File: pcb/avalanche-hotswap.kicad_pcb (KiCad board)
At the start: 2 copper layers, 179.4 x 122.8 mm, 138 parts, among them J1 TRRS, J2 OLED, P1 i2c_pin, P2 i2c_pin, P3 battery+, P4 battery-, SW0 SW_Push, SW1 SW_Push, SW10 SW_Push, SW11 SW_Push, SW12 SW_Push, SW13 SW_Push, SW14 SW_Push, SW15 SW_Push, SW16 SW_Push, SW17 SW_Push, SW18 SW_Push, SW19 SW_Push, SW2 SW_Push, SW20 SW_Push, SW21 SW_Push, SW22 SW_Push, SW23 SW_Push, SW24 SW_Push, SW25 SW_Push, SW26 SW_Push, SW27 SW_Push, SW28 SW_Push, SW29 SW_Push, SW3 SW_Push, SW30 SW_Push, SW31 SW_Push, SW32 SW_Push, SW33 SW_DPDT_x2, SW34 SW_DPDT_x2, SW4 SW_Push, SW5 SW_Push, SW6 SW_Push, SW7 SW_Push, SW8 SW_Push, SW9 SW_Push, U1 ProMicro

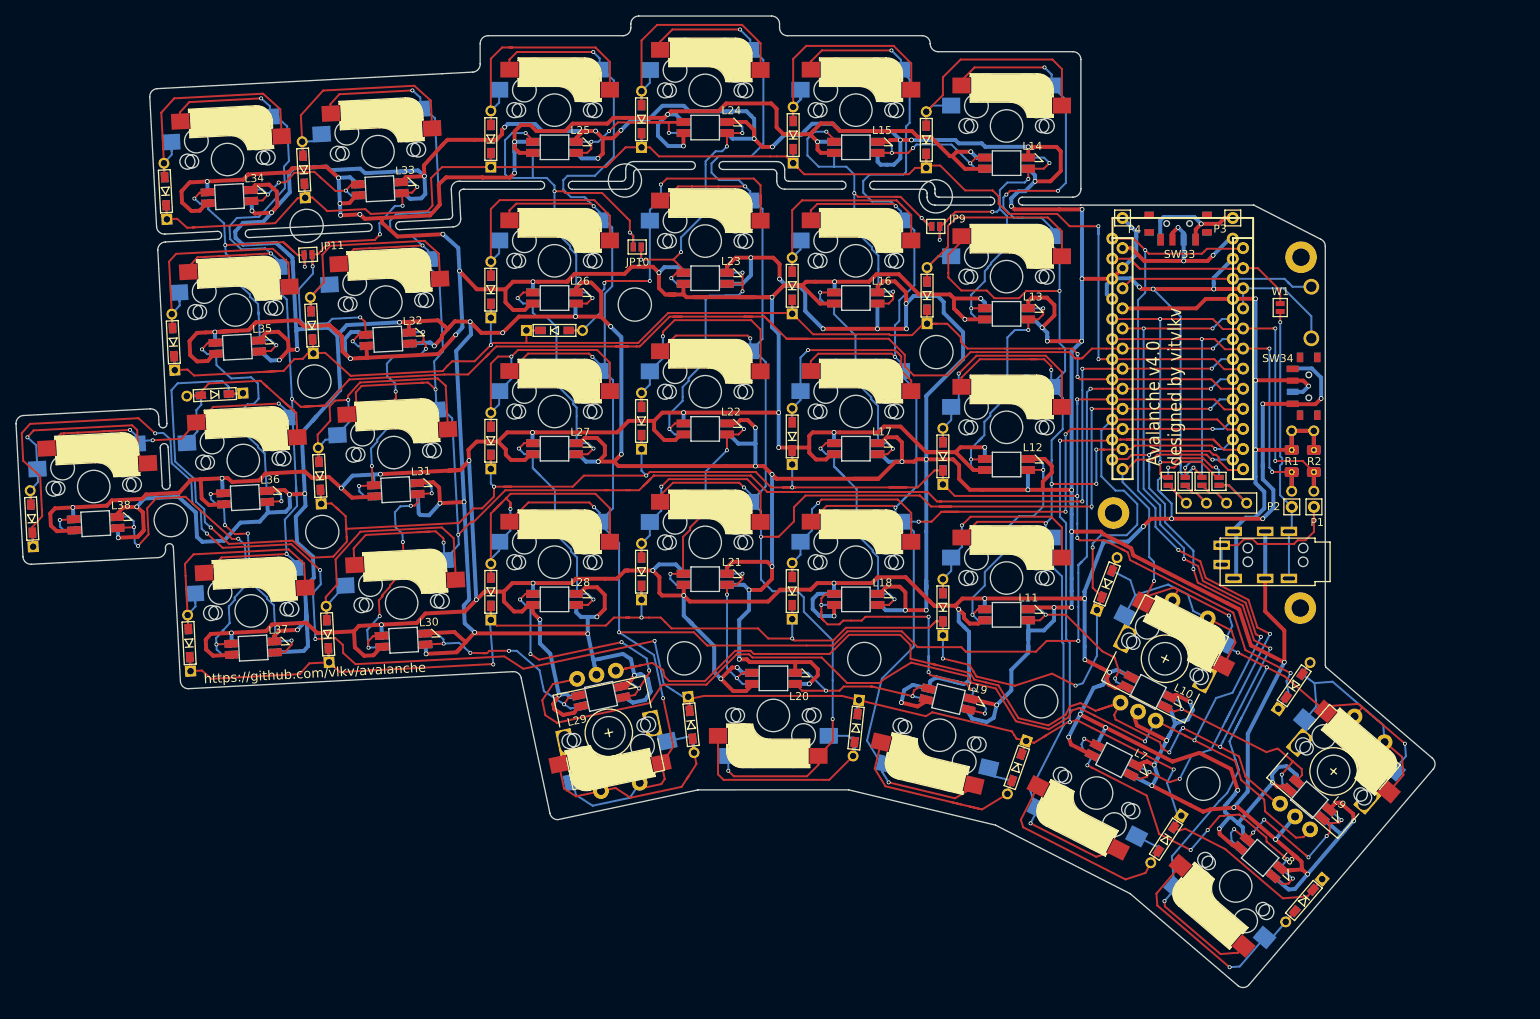
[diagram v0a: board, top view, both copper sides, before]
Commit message: Working on stagger
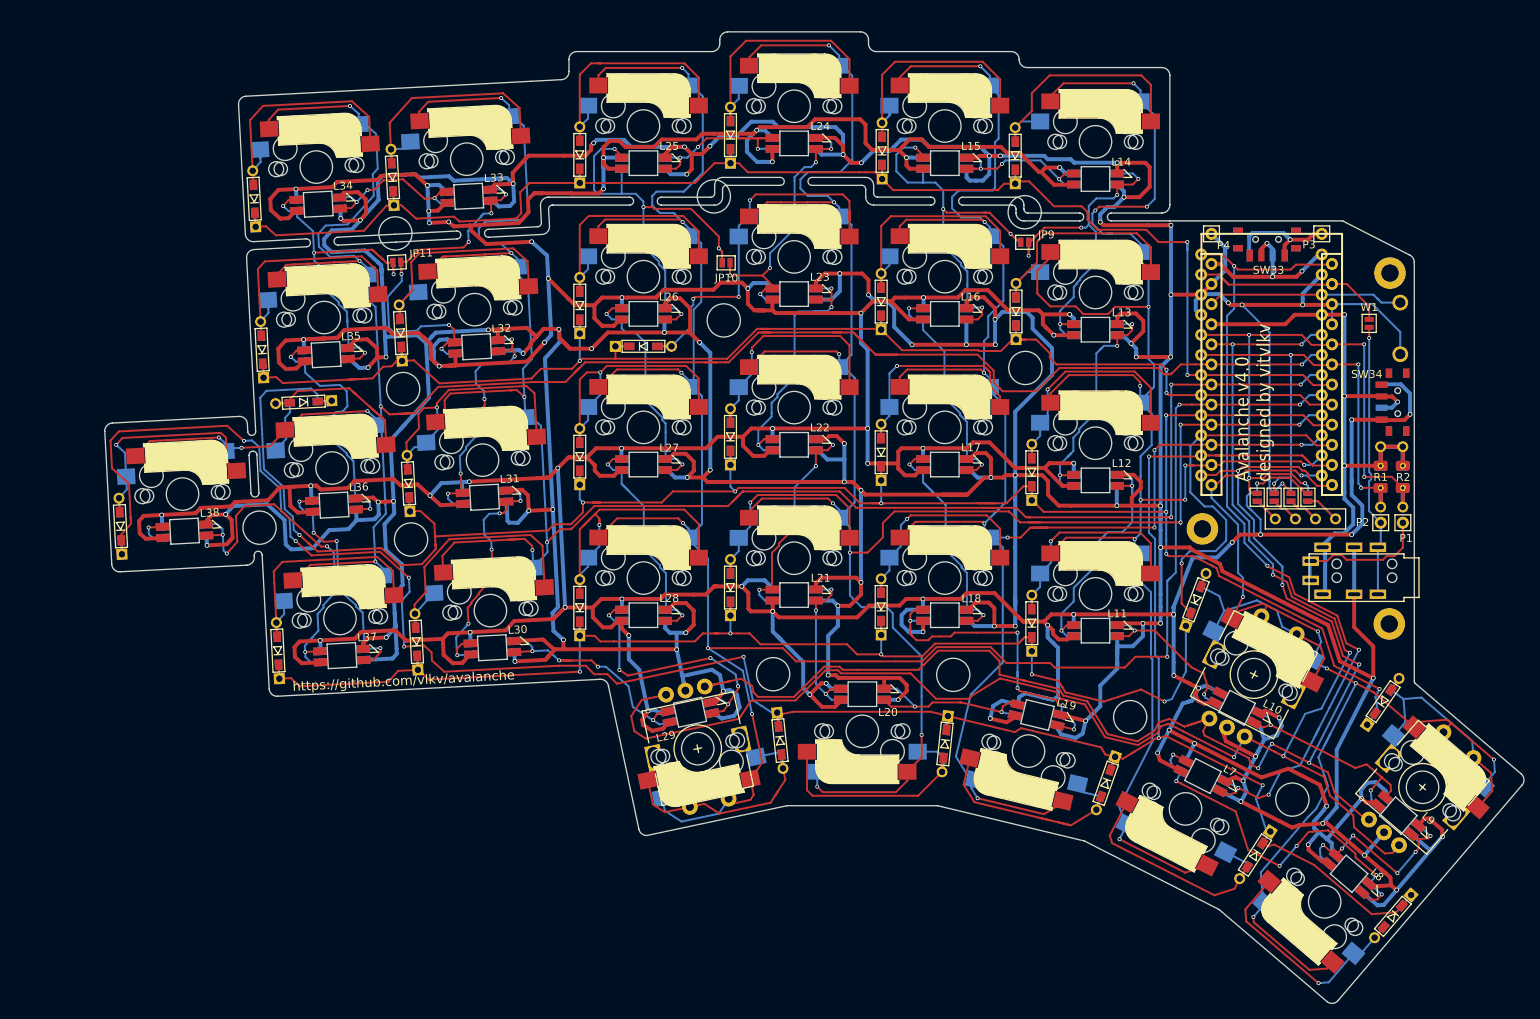
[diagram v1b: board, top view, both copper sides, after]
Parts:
- moved L14 11.4 mm to (162.8, 48.0)
- moved HM14 11.4 mm to (167.2, 116.0)
- moved JP2 11.4 mm to (185.4, 88.2)
- moved L19 11.4 mm to (155.5, 115.8)
- moved L9 11.4 mm to (201.1, 128.5)
- moved D19 11.4 mm to (199.2, 114.1)
- moved J1 11.4 mm to (201.8, 98.4)
- moved JP6 11.4 mm to (185.4, 88.2)
- moved SW11 11.4 mm to (143.8, 60.4)
- moved SW24 11.4 mm to (143.8, 98.5)
- moved SW9 11.4 mm to (105.7, 60.4)
- moved HM10 11.4 mm to (154.0, 71.9)
- moved SW32 11.4 mm to (191.8, 139.4)
- moved D3 11.4 mm to (97.6, 45.0)
- moved HM1 11.4 mm to (200.0, 59.9)
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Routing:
- net GND: track 1144.9 -> 1148.2 mm
- net Net-(L29-Pad2): track 29.9 -> 31.4 mm
- net VCC: track 971.5 -> 970.1 mm
- net row3: track 217.7 -> 216.5 mm
- net row4: track 308.0 -> 308.6 mm
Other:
- outline, holes or cut-outs redrawn

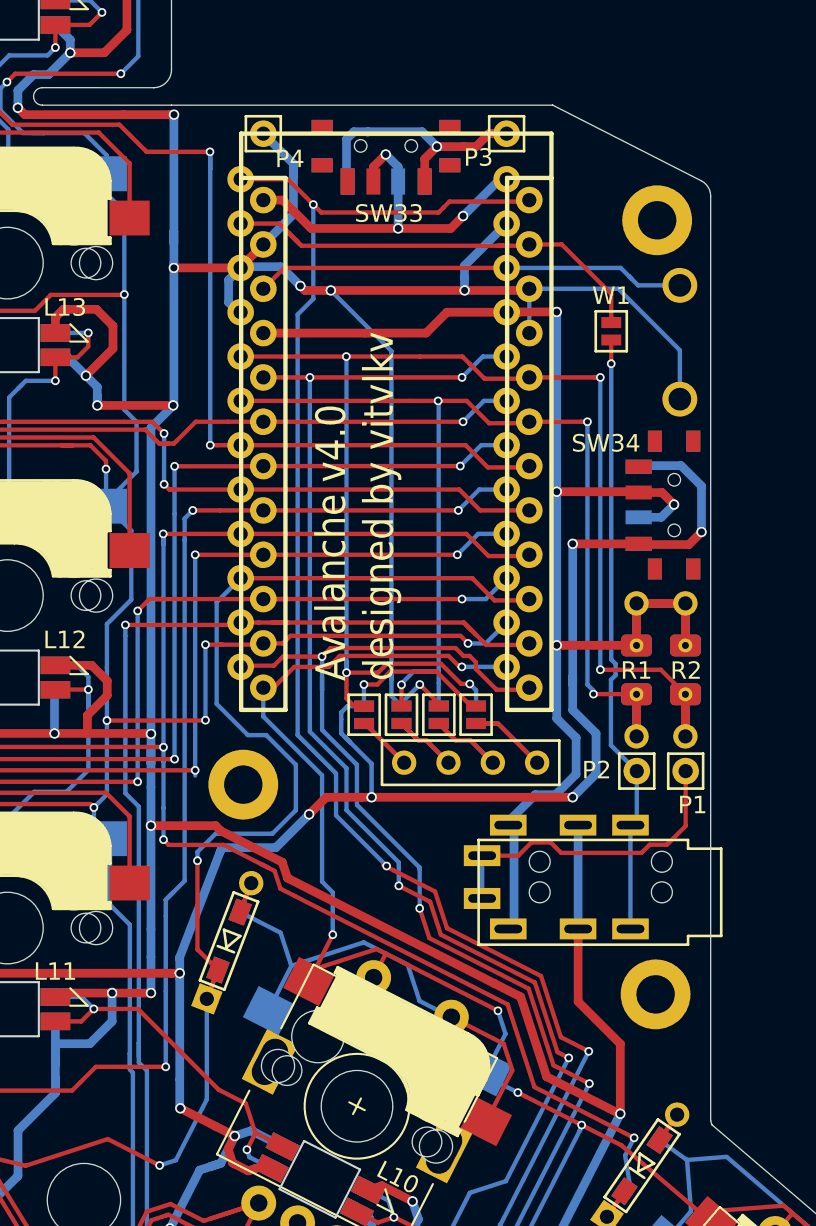
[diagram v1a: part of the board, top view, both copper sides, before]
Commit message: Stagger is done
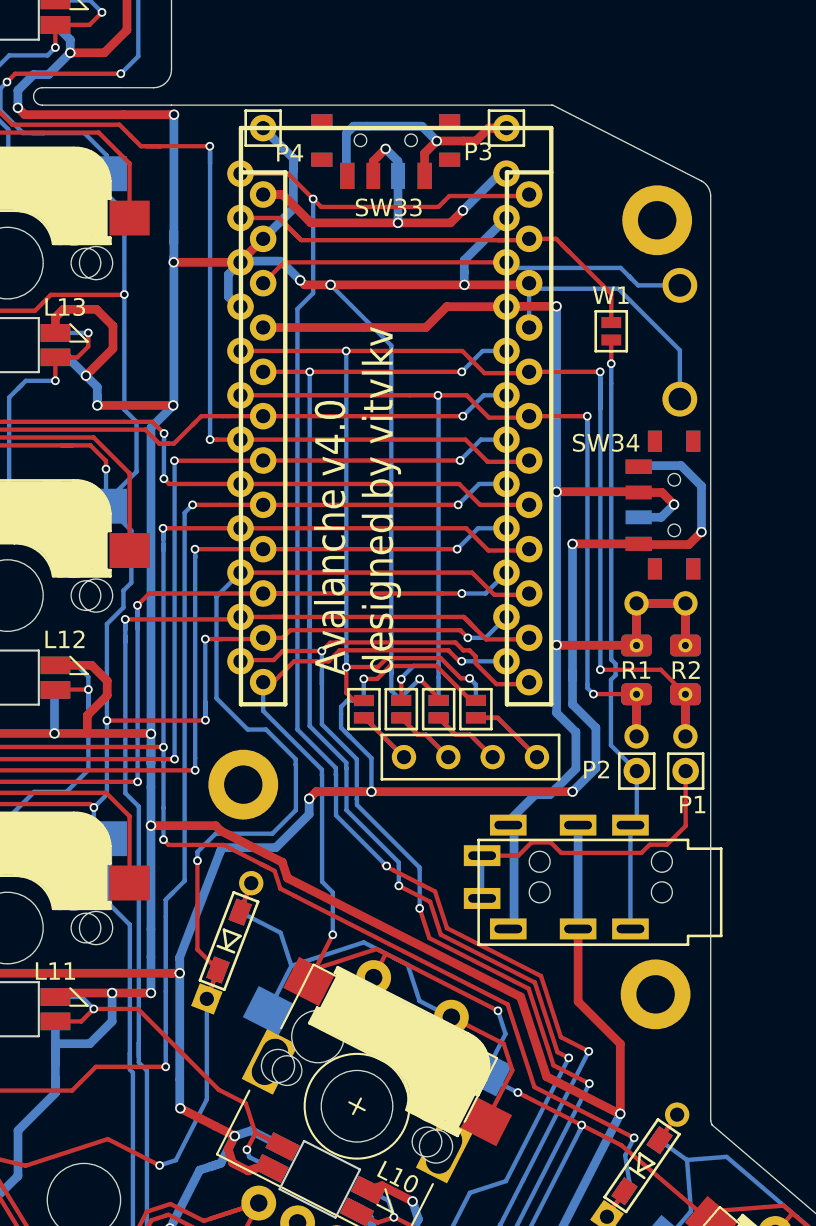
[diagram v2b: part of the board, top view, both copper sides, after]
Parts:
- moved JP6 0.32 mm to (185.4, 87.9)
- moved J2 0.32 mm to (189.4, 90.7)
- moved JP1 0.32 mm to (183.2, 87.9)
- moved JP2 0.32 mm to (185.4, 87.9)
- moved JP4 0.32 mm to (189.7, 87.9)
- moved JP8 0.32 mm to (189.7, 87.9)
- moved U1 0.32 mm to (185.0, 72.0)
- moved P4 0.32 mm to (177.5, 54.6)
- moved SW33 0.32 mm to (184.5, 55.3)
- moved P3 0.32 mm to (191.4, 54.6)
- moved JP7 0.32 mm to (187.5, 87.9)
- moved JP3 0.32 mm to (187.5, 87.9)
- moved JP5 0.32 mm to (183.2, 87.9)
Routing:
- net SDA: track 78.5 -> 80.6 mm
- net col4: track 231.1 -> 232.5 mm
- net row4: track 308.6 -> 309.9 mm
- net row2: track 271.2 -> 272.5 mm
- net VCC: track 970.1 -> 971.2 mm
- net col5: track 221.3 -> 222.4 mm
- net SCL: track 64.7 -> 65.7 mm
- net DATA: track 26.9 -> 27.6 mm
- net row0: track 190.8 -> 191.4 mm
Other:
- outline, holes or cut-outs redrawn
